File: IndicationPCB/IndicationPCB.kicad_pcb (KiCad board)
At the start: 2 copper layers, 12.5 x 63.5 mm, 14 parts, among them J1 Conn_01x03

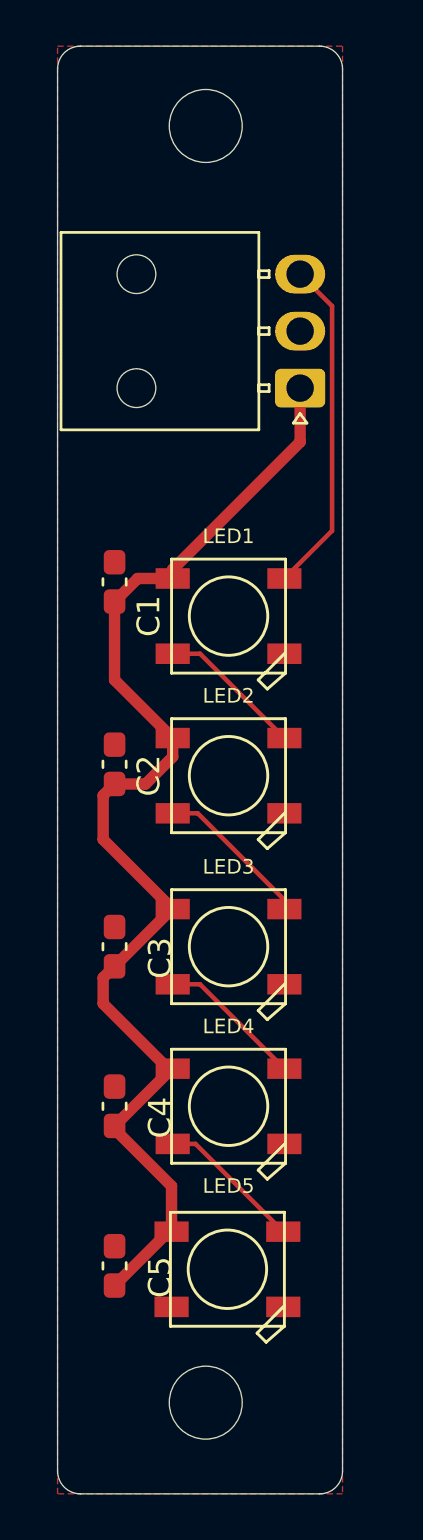
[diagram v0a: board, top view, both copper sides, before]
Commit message: fixed
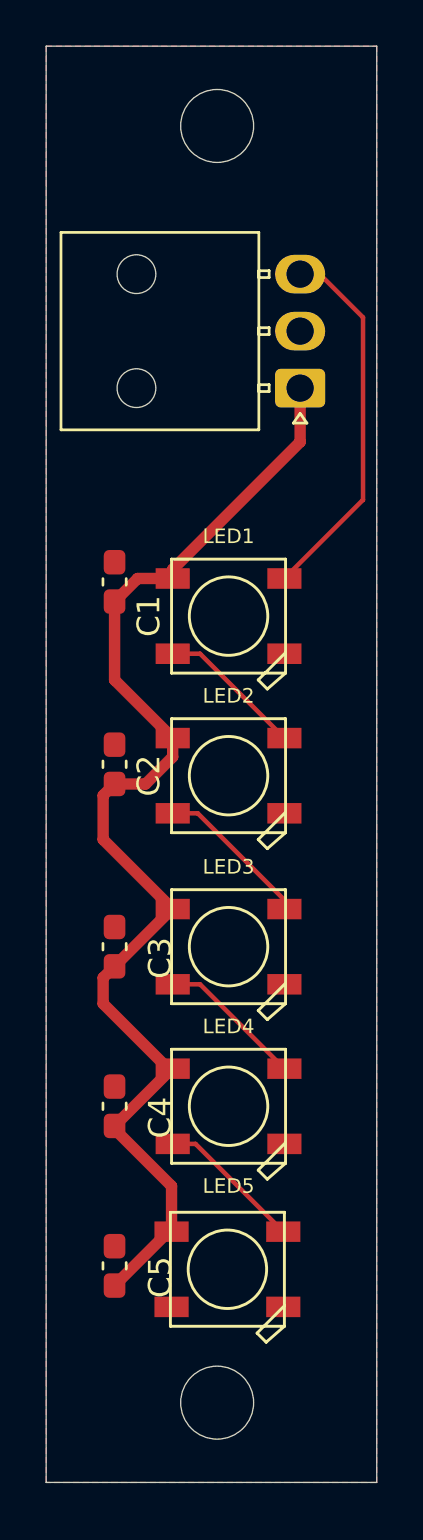
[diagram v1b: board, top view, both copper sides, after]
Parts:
- moved H1 0.50 mm to (144.5, 52.0)
- moved H2 0.50 mm to (144.5, 108.0)
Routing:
- net /DIN: track 14.8 -> 16.4 mm
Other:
- board size 12.5 x 63.5 mm -> 14.5 x 63 mm
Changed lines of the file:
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@@
 	(footprint "MountingHole:MountingHole_3.2mm_M3"
 		(layer "F.Cu")
-		(at 144 52)
+		(at 144.5 52)
 		(descr "Mounting Hole 3.2mm, no annular, M3")
 		(tags "mounting hole 3.2mm no annular m3")
@@
 	(footprint "MountingHole:MountingHole_3.2mm_M3"
 		(layer "F.Cu")
-		(at 144 108)
+		(at 144.5 108)
 		(descr "Mounting Hole 3.2mm, no annular, M3")
 		(tags "mounting hole 3.2mm no annular m3")
@@
 		(embedded_fonts no)
 	)
-	(gr_arc
-		(start 138.5 112)
-		(mid 137.792893 111.707107)
-		(end 137.5 111)
+	(gr_rect
+		(start 137 48.5)
+		(end 151.5 111.5)
 		(stroke
 			(width 0.05)
 			(type default)
 		)
-		(layer "Edge.Cuts")
-	)
-	(gr_arc
-		(start 149 48.5)
-		(mid 149.707107 48.792893)
-		(end 150 49.5)
-		(stroke
-			(width 0.05)
-			(type default)
-		)
-		(layer "Edge.Cuts")
-	)
-	(gr_line
-		(start 137.5 111)
-		(end 137.5 49.5)
-		(stroke
-			(width 0.05)
-			(type default)
-		)
-		(layer "Edge.Cuts")
-	)
-	(gr_line
-		(start 150 49.5)
-		(end 150 111)
-		(stroke
-			(width 0.05)
-			(type default)
-		)
-		(layer "Edge.Cuts")
-	)
-	(gr_line
-		(start 138.5 48.5)
-		(end 149 48.5)
-		(stroke
-			(width 0.05)
-			(type default)
-		)
-		(layer "Edge.Cuts")
-	)
-	(gr_line
-		(start 149 112)
-		(end 138.5 112)
-		(stroke
-			(width 0.05)
-			(type default)
-		)
-		(layer "Edge.Cuts")
-	)
-	(gr_arc
-		(start 137.5 49.5)
-		(mid 137.792893 48.792893)
-		(end 138.5 48.5)
-		(stroke
-			(width 0.05)
-			(type default)
-		)
-		(layer "Edge.Cuts")
-	)
-	(gr_arc
-		(start 150 111)
-		(mid 149.707107 111.707107)
-		(end 149 112)
-		(stroke
-			(width 0.05)
-			(type default)
-		)
+		(fill no)
 		(layer "Edge.Cuts")
 	)
@@
 	(segment
 		(start 147.45 71.85)
-		(end 149.541 69.759)
+		(end 150.899 68.401)
 		(width 0.2)
 		(layer "F.Cu")
@@
 	)
 	(segment
-		(start 149.541 69.759)
-		(end 149.541 59.901)
+		(start 150.899 60.399)
+		(end 149 58.5)
 		(width 0.2)
 		(layer "F.Cu")
@@
 	)
 	(segment
-		(start 149.541 59.901)
+		(start 149 58.5)
 		(end 148.14 58.5)
+		(width 0.2)
+		(layer "F.Cu")
+		(net 3)
+	)
+	(segment
+		(start 150.899 68.401)
+		(end 150.899 60.399)
 		(width 0.2)
 		(layer "F.Cu")
@@
 		(polygon
 			(pts
-				(xy 137.5 48.5) (xy 150 48.5) (xy 150 112) (xy 137.5 112)
-			)
-		)
+				(xy 137 48.5) (xy 151.5 48.5) (xy 151.5 111.5) (xy 137 111.5)
+			)
+		)
